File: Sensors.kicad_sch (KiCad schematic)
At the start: 16 parts, among them U6 AS333

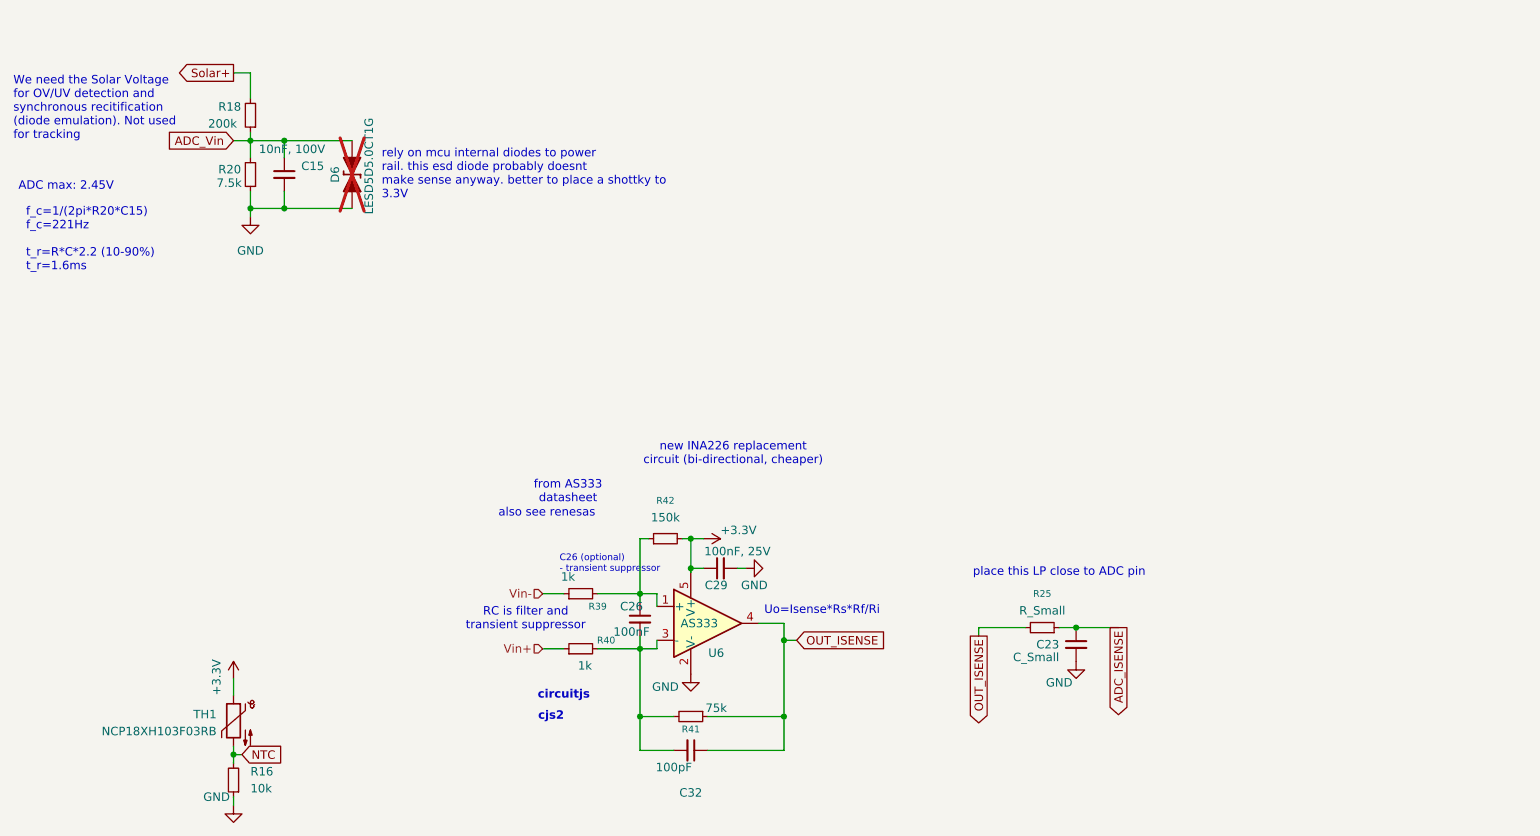
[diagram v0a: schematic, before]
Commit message: restored INA226 schematics
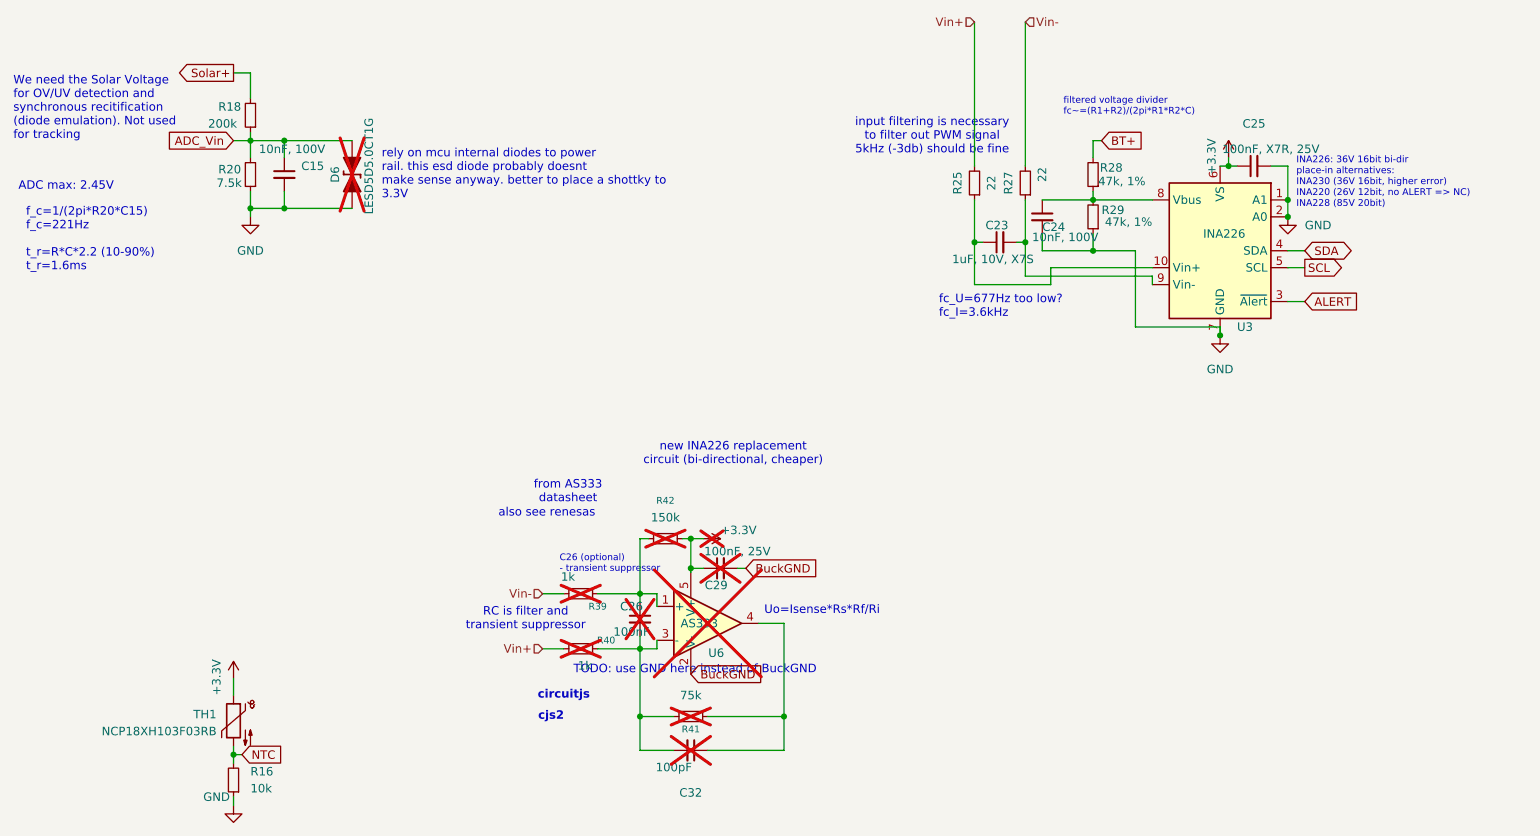
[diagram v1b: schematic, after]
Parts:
- added C24: 10nF, 100V, Capacitor_SMD:C_0805_2012Metric, symbol Device:C_Small
- added C25: 100nF, X7R, 25V, Capacitor_SMD:C_0805_2012Metric, symbol Device:C_Small
- added R27: 22, Resistor_SMD:R_0805_2012Metric, symbol Device:R_Small
- added R28, R29: 47k, 1%, Resistor_SMD:R_0805_2012Metric, symbol Device:R_Small
- added U3: INA226, Package_SO:VSSOP-10_3x3mm_P0.5mm, symbol Sensor_Energy:INA226
- C23: value C_Small -> 1uF, 10V, X7S; Desc (none) -> CS_Filt; Digikey (none) -> CL21B105KAFNNNE; MPN (none) -> 1uF, 10V, X7S
- C26, C29, C32, R39, R40, R41, R42, U6: now not fitted
- R25: value R_Small -> 22; footprint Resistor_SMD:R_0805_2012Metric_Pad1.20x1.40mm_HandSolder -> Resistor_SMD:R_0805_2012Metric; Desc (none) -> CS_FILT; MPN (none) -> 22
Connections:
- net +3.3V: now also C25.1, U3.6 (VS)
- net GND: now also C24.2, C25.2, R29.1, U3.1 (A1), U3.2 (A0), U3.7 (GND); no longer C23.2, C29.2, U6.2 (V-)
- net Vin+: now also R25.2
- net Vin-: now also R27.2
- net ADC_ISENSE: no longer names the net of C23.1, R25.1
- net ADC_ISENSE: now also U3.10 (Vin+)
- net OUT_ISENSE: no longer names the net of C32.1, R41.1, U6.4
- net OUT_ISENSE: no longer R25.2
- new net: C23.2, R27.1, U3.9 (Vin-)
- new net: C24.1, R28.1, R29.2, U3.8 (Vbus)
- new net ALERT: U3.3 (~{Alert})
- new net BT+: R28.2
- new net BuckGND: C29.2, U6.2 (V-)
- new net SCL: U3.5 (SCL)
- new net SDA: U3.4 (SDA)
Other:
- note added: "INA226: 36V 16bit bi-dir place-in alternatives: INA230 (36V 16bit, higher error) INA220 (26V 12bit, no ALERT => NC) INA228 (85V 20bit)"
- note added: "TODO: use GND here instead of BuckGND"
- note added: "fc_U=677Hz too low? fc_I=3.6kHz"
- note added: "filtered voltage divider fc~=(R1+R2)/(2pi*R1*R2*C)"
- note added: "input filtering is necessary to filter out PWM signal 5kHz (-3db) should be fine"
- note removed: "place this LP close to ADC pin"
